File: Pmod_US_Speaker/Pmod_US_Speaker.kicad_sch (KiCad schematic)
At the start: 2 parts, among them IC1 IR4427STRPBF, U1 CUSA-T80-18-2400-TH

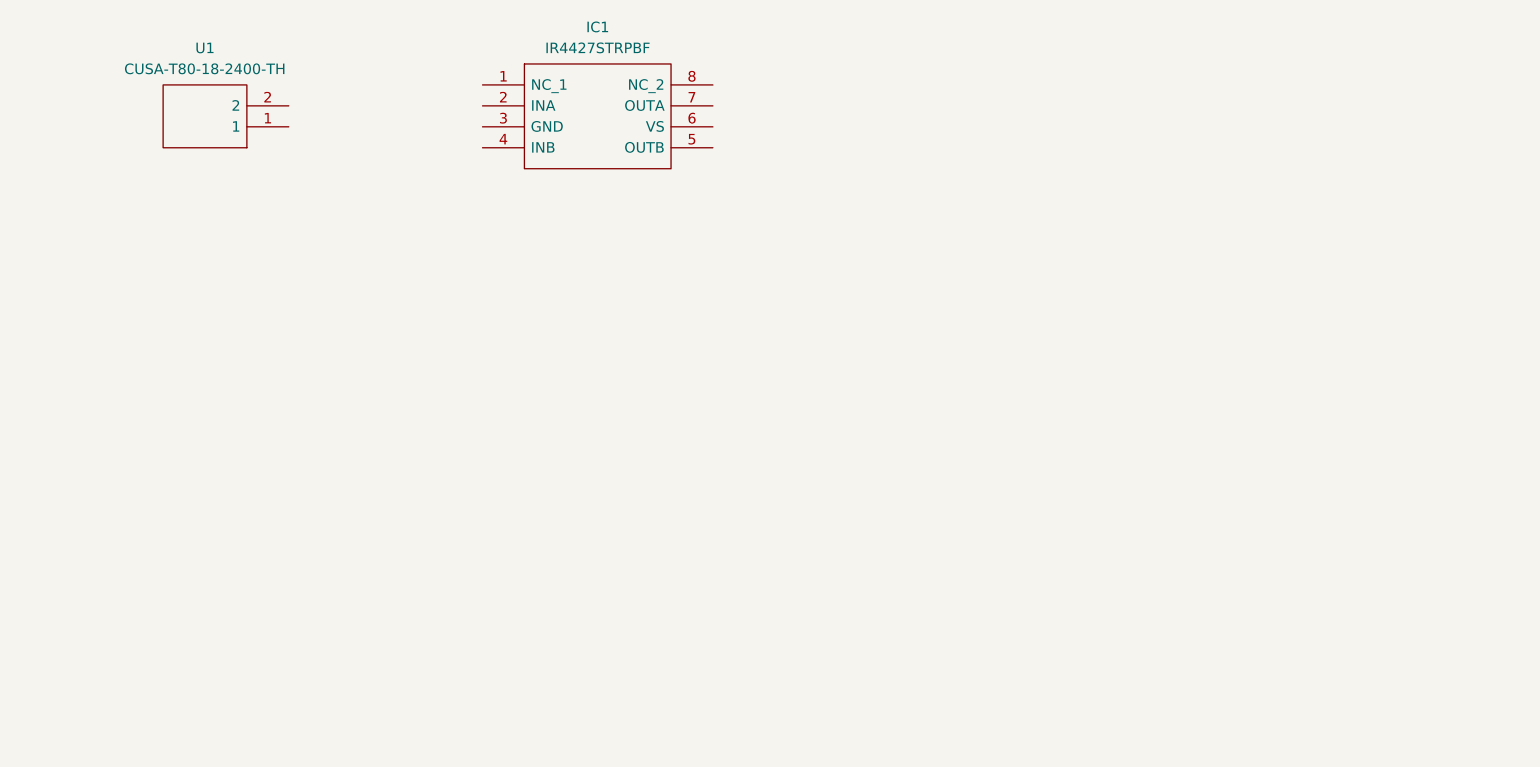
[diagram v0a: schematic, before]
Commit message: 1027
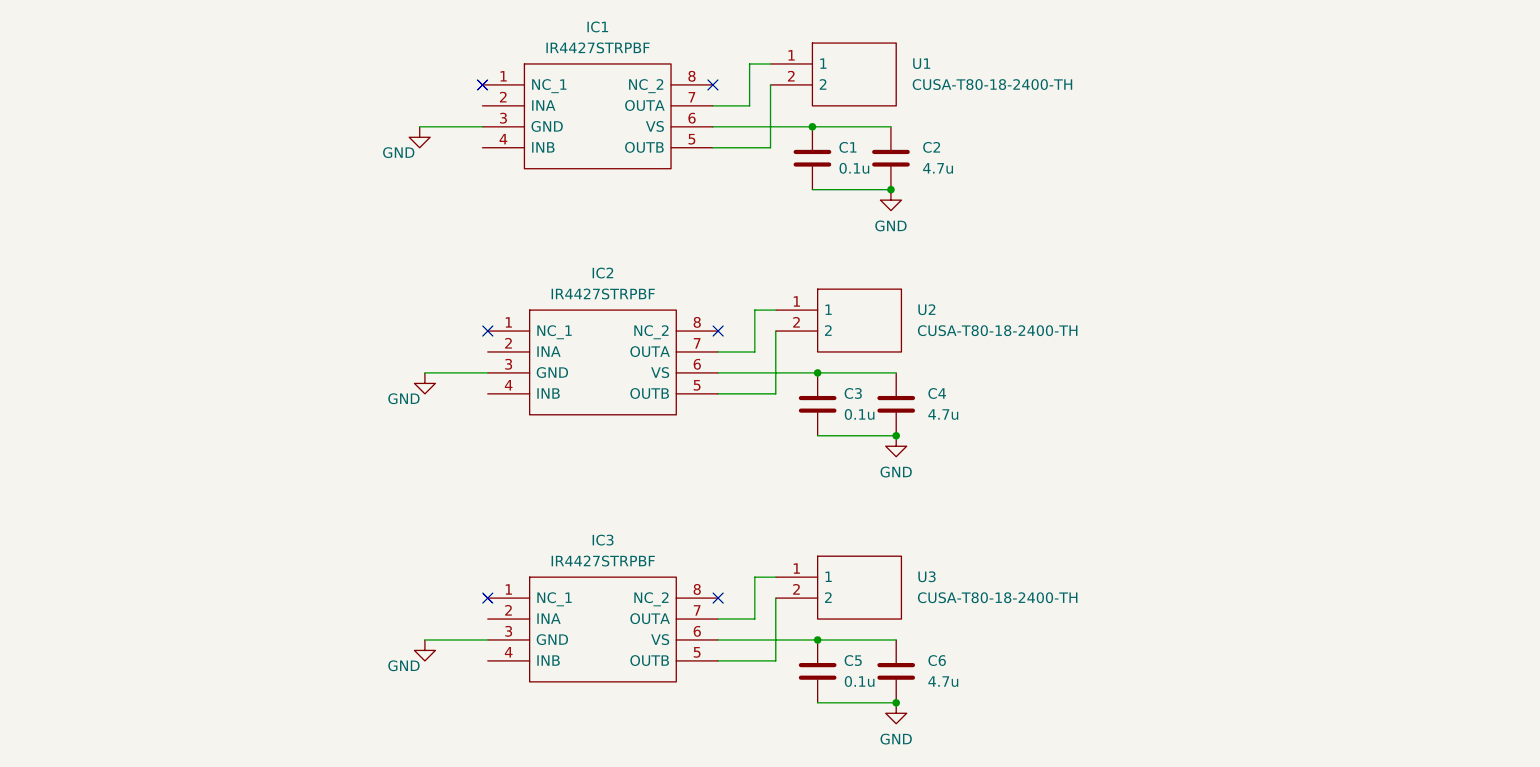
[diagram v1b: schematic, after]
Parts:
- added C1, C3, C5: 0.1u, Capacitor_SMD:C_0603_1608Metric_Pad1.08x0.95mm_HandSolder, symbol Device:C
- added C2, C4, C6: 4.7u, Capacitor_SMD:C_0805_2012Metric_Pad1.18x1.45mm_HandSolder, symbol Device:C
- added IC2, IC3: IR4427STRPBF, SOIC127P600X175-8N, symbol samacsys:IR4427STRPBF
- added U2, U3: CUSA-T80-18-2400-TH, CUSAT80182400TH, symbol samacsys:CUSA-T80-18-2400-TH
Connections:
- net GND: now reaches IC1.3 (GND)
- net GND: now also C1.2, C2.2, C3.2, C4.2, C5.2, C6.2, IC2.3 (GND), IC3.3 (GND)
- net at IC1.5 (OUTB): now also U1.2
- net at IC1.6 (VS): now also C1.1, C2.1
- net at IC1.7 (OUTA): now also U1.1
- new net: IC2.5 (OUTB), U2.2
- new net: C3.1, C4.1, IC2.6 (VS)
- new net: IC2.7 (OUTA), U2.1
- new net: IC3.5 (OUTB), U3.2
- new net: C5.1, C6.1, IC3.6 (VS)
- new net: IC3.7 (OUTA), U3.1
- no-connect marks 0 -> 6
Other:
- moved on the sheet: U1

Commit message: 1028
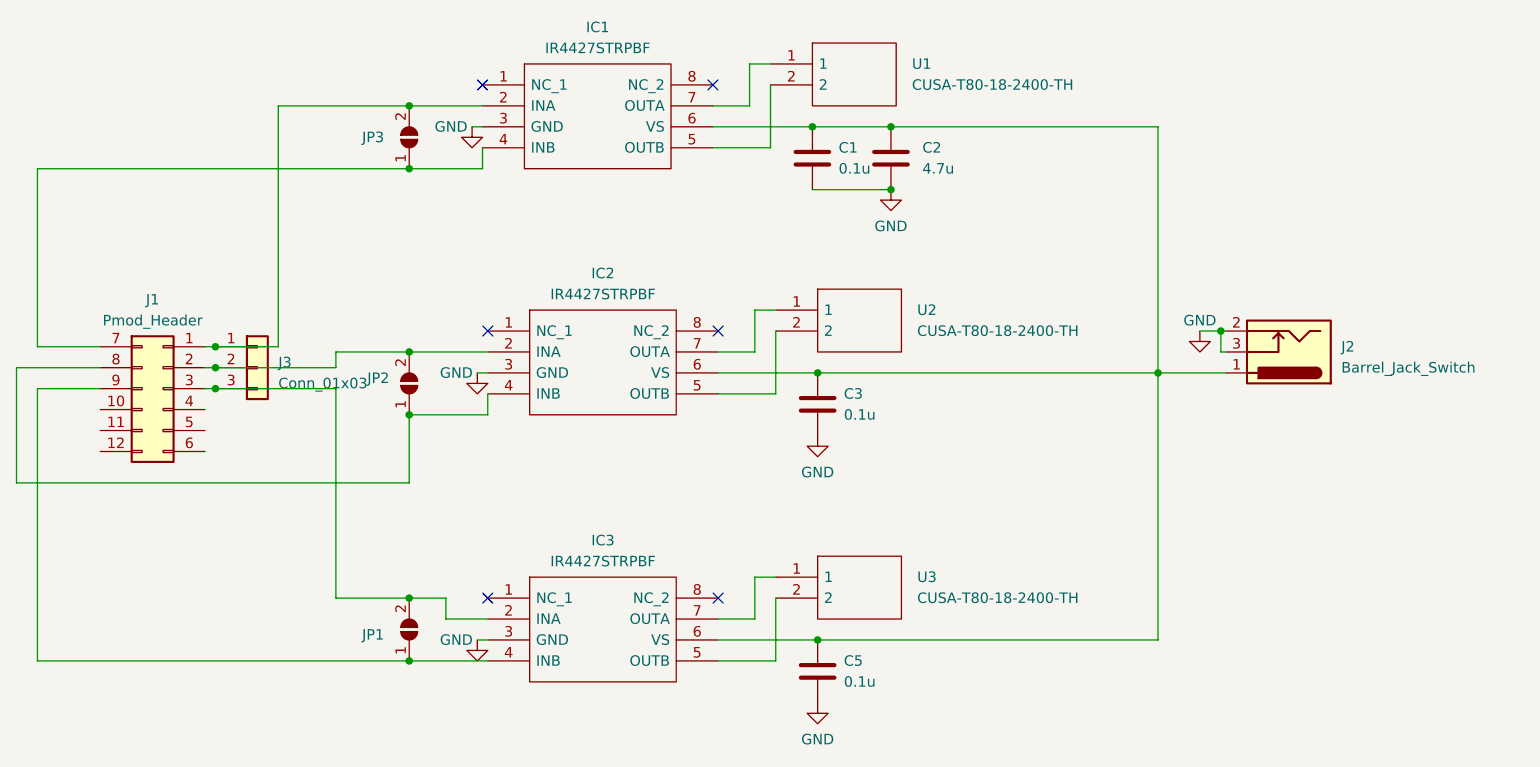
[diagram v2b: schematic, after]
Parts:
- removed C4, C6: 4.7u, Capacitor_SMD:C_0805_2012Metric_Pad1.18x1.45mm_HandSolder, symbol Device:C
- added J1: Pmod_Header, Connector_PinHeader_2.54mm:PinHeader_2x06_P2.54mm_Vertical, symbol MyLibrary:Pmod_Header
- added J2: Barrel_Jack_Switch, Connector_BarrelJack:BarrelJack_CUI_PJ-036AH-SMT_Horizontal, symbol Connector:Barrel_Jack_Switch
- added J3: Conn_01x03, Connector_PinHeader_2.54mm:PinHeader_1x03_P2.54mm_Vertical, symbol Connector_Generic:Conn_01x03
- added JP1: SolderJumper_2_Open, Jumper:SolderJumper-2_P1.3mm_Open_TrianglePad1.0x1.5mm, symbol Jumper:SolderJumper_2_Open
- added JP2, JP3: SolderJumper_2_Open, symbol Jumper:SolderJumper_2_Open
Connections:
- net GND: now also J2.2, J2.3
- net at C1.1, C2.1, IC1.6 (VS): now also C3.1, C5.1, IC2.6 (VS), IC3.6 (VS), J2.1
- net at IC2.2 (INA): now also J1.2 (Pin_2), J3.2 (Pin_2), JP2.2 (B)
- net at IC2.4 (INB): now also J1.8 (Pin_8), JP2.1 (A)
- net at IC1.2 (INA): now also J1.1 (Pin_1), J3.1 (Pin_1), JP3.2 (B)
- net at IC1.4 (INB): now also J1.7 (Pin_7), JP3.1 (A)
- net at IC3.2 (INA): now also J1.3 (Pin_3), J3.3 (Pin_3), JP1.2 (B)
- net at IC3.4 (INB): now also J1.9 (Pin_9), JP1.1 (A)

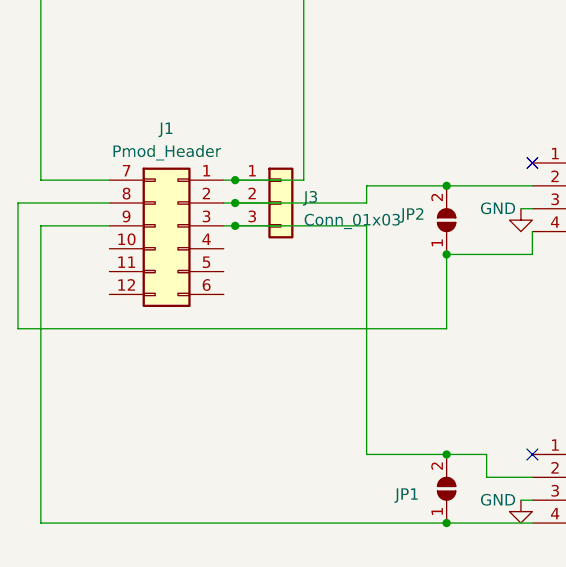
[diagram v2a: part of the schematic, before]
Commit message: 1028
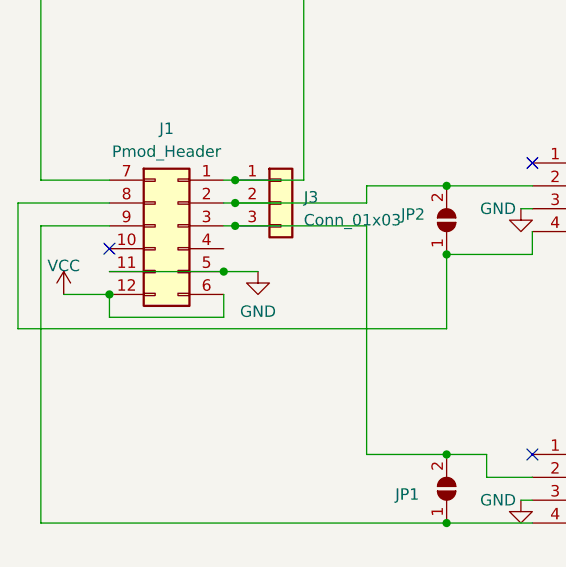
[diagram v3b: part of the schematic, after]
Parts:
- IC1, IC2, IC3: footprint SOIC127P600X175-8N -> SamacSys_Parts:SOIC127P600X175-8N
- JP2, JP3: footprint (none) -> Jumper:SolderJumper-2_P1.3mm_Open_TrianglePad1.0x1.5mm
- U1, U2, U3: footprint CUSAT80182400TH -> SamacSys_Parts:CUSAT80182400TH
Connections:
- net GND: now also J1.11 (Pin_11), J1.5 (Pin_5)
- net VCC: now reaches J1.12 (Pin_12)
- net VCC: now also J1.6 (Pin_6)
- no-connect marks 6 -> 7
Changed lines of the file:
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@@
   (junction (at 176.53 101.6) (diameter 0) (color 0 0 0 0)
   )
+  (junction (at 53.34 113.665) (diameter 0) (color 0 0 0 0)
+  )
   (junction (at 127.635 139.065) (diameter 0) (color 0 0 0 0)
   )
@@
   )
   (junction (at 78.105 74.295) (diameter 0) (color 0 0 0 0)
+  )
+  (junction (at 40.64 116.205) (diameter 0) (color 0 0 0 0)
   )
   (junction (at 78.105 141.605) (diameter 0) (color 0 0 0 0)
@@
   (no_connect (at 87.63 133.985))
   (no_connect (at 115.57 101.6))
+  (no_connect (at 40.64 111.125))
   (no_connect (at 115.57 133.985))
   (no_connect (at 114.935 71.755))
@@
     (stroke (width 0) (type default))
   )
+  (wire (pts (xy 53.34 113.665) (xy 57.15 113.665))
+    (stroke (width 0) (type default))
+  )
   (wire (pts (xy 114.935 79.375) (xy 121.92 79.375))
     (stroke (width 0) (type default))
@@
     (stroke (width 0) (type default))
   )
+  (wire (pts (xy 40.64 116.205) (xy 40.64 118.745))
+    (stroke (width 0) (type default))
+  )
   (wire (pts (xy 40.64 108.585) (xy 33.02 108.585))
     (stroke (width 0) (type default))
@@
     (stroke (width 0) (type default))
   )
+  (wire (pts (xy 40.64 113.665) (xy 53.34 113.665))
+    (stroke (width 0) (type default))
+  )
   (wire (pts (xy 82.55 136.525) (xy 87.63 136.525))
     (stroke (width 0) (type default))
@@
     (stroke (width 0) (type default))
   )
+  (wire (pts (xy 35.56 116.205) (xy 40.64 116.205))
+    (stroke (width 0) (type default))
+  )
   (wire (pts (xy 120.015 99.06) (xy 122.555 99.06))
     (stroke (width 0) (type default))
@@
     (stroke (width 0) (type default))
   )
+  (wire (pts (xy 53.34 118.745) (xy 53.34 116.205))
+    (stroke (width 0) (type default))
+  )
   (wire (pts (xy 78.105 133.985) (xy 82.55 133.985))
     (stroke (width 0) (type default))
   )
   (wire (pts (xy 127 84.455) (xy 136.525 84.455))
+    (stroke (width 0) (type default))
+  )
+  (wire (pts (xy 40.64 118.745) (xy 53.34 118.745))
     (stroke (width 0) (type default))
   )
@@
       (effects (font (size 1.27 1.27)) (justify right) hide)
     )
-    (property "Footprint" "" (at 78.105 107.95 0)
+    (property "Footprint" "Jumper:SolderJumper-2_P1.3mm_Open_TrianglePad1.0x1.5mm" (at 78.105 107.95 0)
       (effects (font (size 1.27 1.27)) hide)
     )
@@
     )
   )
+  (symbol (lib_id "power:GND") (at 57.15 113.665 0) (unit 1)
+    (in_bom yes) (on_board yes) (dnp no) (fields_autoplaced)
+    (property "Reference" "#PWR09" (at 57.15 120.015 0)
+      (effects (font (size 1.27 1.27)) hide)
+    )
+    (property "Value" "GND" (at 57.15 118.11 0)
+      (effects (font (size 1.27 1.27)))
+    )
+    (property "Footprint" "" (at 57.15 113.665 0)
+      (effects (font (size 1.27 1.27)) hide)
+    )
+    (property "Datasheet" "" (at 57.15 113.665 0)
+      (effects (font (size 1.27 1.27)) hide)
+    )
+    (pin "1")
+    (instances
+      (project "Pmod_US_Speaker"
+        (path "/03748716-5307-454c-bec9-0fb4b0acd2b9"
+          (reference "#PWR09") (unit 1)
+        )
+      )
+    )
+  )
   (symbol (lib_id "samacsys:IR4427STRPBF") (at 87.63 101.6 0) (unit 1)
     (in_bom yes) (on_board yes) (dnp no) (fields_autoplaced)
@@
       (effects (font (size 1.27 1.27)))
     )
-    (property "Footprint" "SOIC127P600X175-8N" (at 111.76 99.06 0)
+    (property "Footprint" "SamacSys_Parts:SOIC127P600X175-8N" (at 111.76 99.06 0)
       (effects (font (size 1.27 1.27)) (justify left) hide)
     )
@@
       (effects (font (size 1.27 1.27)))
     )
-    (property "Footprint" "SOIC127P600X175-8N" (at 111.125 69.215 0)
+    (property "Footprint" "SamacSys_Parts:SOIC127P600X175-8N" (at 111.125 69.215 0)
       (effects (font (size 1.27 1.27)) (justify left) hide)
     )
@@
       (effects (font (size 1.27 1.27)) (justify left))
     )
-    (property "Footprint" "CUSAT80182400TH" (at 139.065 96.52 0)
+    (property "Footprint" "SamacSys_Parts:CUSAT80182400TH" (at 139.065 96.52 0)
       (effects (font (size 1.27 1.27)) (justify left) hide)
     )
@@
         (path "/03748716-5307-454c-bec9-0fb4b0acd2b9"
           (reference "U2") (unit 1)
+        )
+      )
+    )
+  )
+  (symbol (lib_id "power:VCC") (at 35.56 116.205 0) (unit 1)
+    (in_bom yes) (on_board yes) (dnp no) (fields_autoplaced)
+    (property "Reference" "#PWR08" (at 35.56 120.015 0)
+      (effects (font (size 1.27 1.27)) hide)
+    )
+    (property "Value" "VCC" (at 35.56 113.03 0)
+      (effects (font (size 1.27 1.27)))
+    )
+    (property "Footprint" "" (at 35.56 116.205 0)
+      (effects (font (size 1.27 1.27)) hide)
+    )
+    (property "Datasheet" "" (at 35.56 116.205 0)
+      (effects (font (size 1.27 1.27)) hide)
+    )
+    (pin "1")
+    (instances
+      (project "Pmod_US_Speaker"
+        (path "/03748716-5307-454c-bec9-0fb4b0acd2b9"
+          (reference "#PWR08") (unit 1)
         )
       )
@@
       (effects (font (size 1.27 1.27)) (justify right) hide)
     )
-    (property "Footprint" "" (at 78.105 78.105 0)
+    (property "Footprint" "Jumper:SolderJumper-2_P1.3mm_Open_TrianglePad1.0x1.5mm" (at 78.105 78.105 0)
       (effects (font (size 1.27 1.27)) hide)
     )
@@
       (effects (font (size 1.27 1.27)) (justify left))
     )
-    (property "Footprint" "CUSAT80182400TH" (at 138.43 66.675 0)
+    (property "Footprint" "SamacSys_Parts:CUSAT80182400TH" (at 138.43 66.675 0)
       (effects (font (size 1.27 1.27)) (justify left) hide)
     )
@@
       (effects (font (size 1.27 1.27)))
     )
-    (property "Footprint" "SOIC127P600X175-8N" (at 111.76 131.445 0)
+    (property "Footprint" "SamacSys_Parts:SOIC127P600X175-8N" (at 111.76 131.445 0)
       (effects (font (size 1.27 1.27)) (justify left) hide)
     )
@@
       (effects (font (size 1.27 1.27)) (justify left))
     )
-    (property "Footprint" "CUSAT80182400TH" (at 139.065 128.905 0)
-      (effects (font (size 1.27 1.27)) (justify left) hide)
-    )
+    (property "Footprint" "SamacSys_Parts:CUSAT80182400TH" (at 139.065 128.905 0)
+      (effects (font (size 1.27 1.27)) (justify left) hide)
+    )
